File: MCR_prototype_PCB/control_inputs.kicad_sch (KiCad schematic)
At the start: 67 parts, among them J4 Conn_01x19_Pin, U1 74AHC165, U2 74AHC165

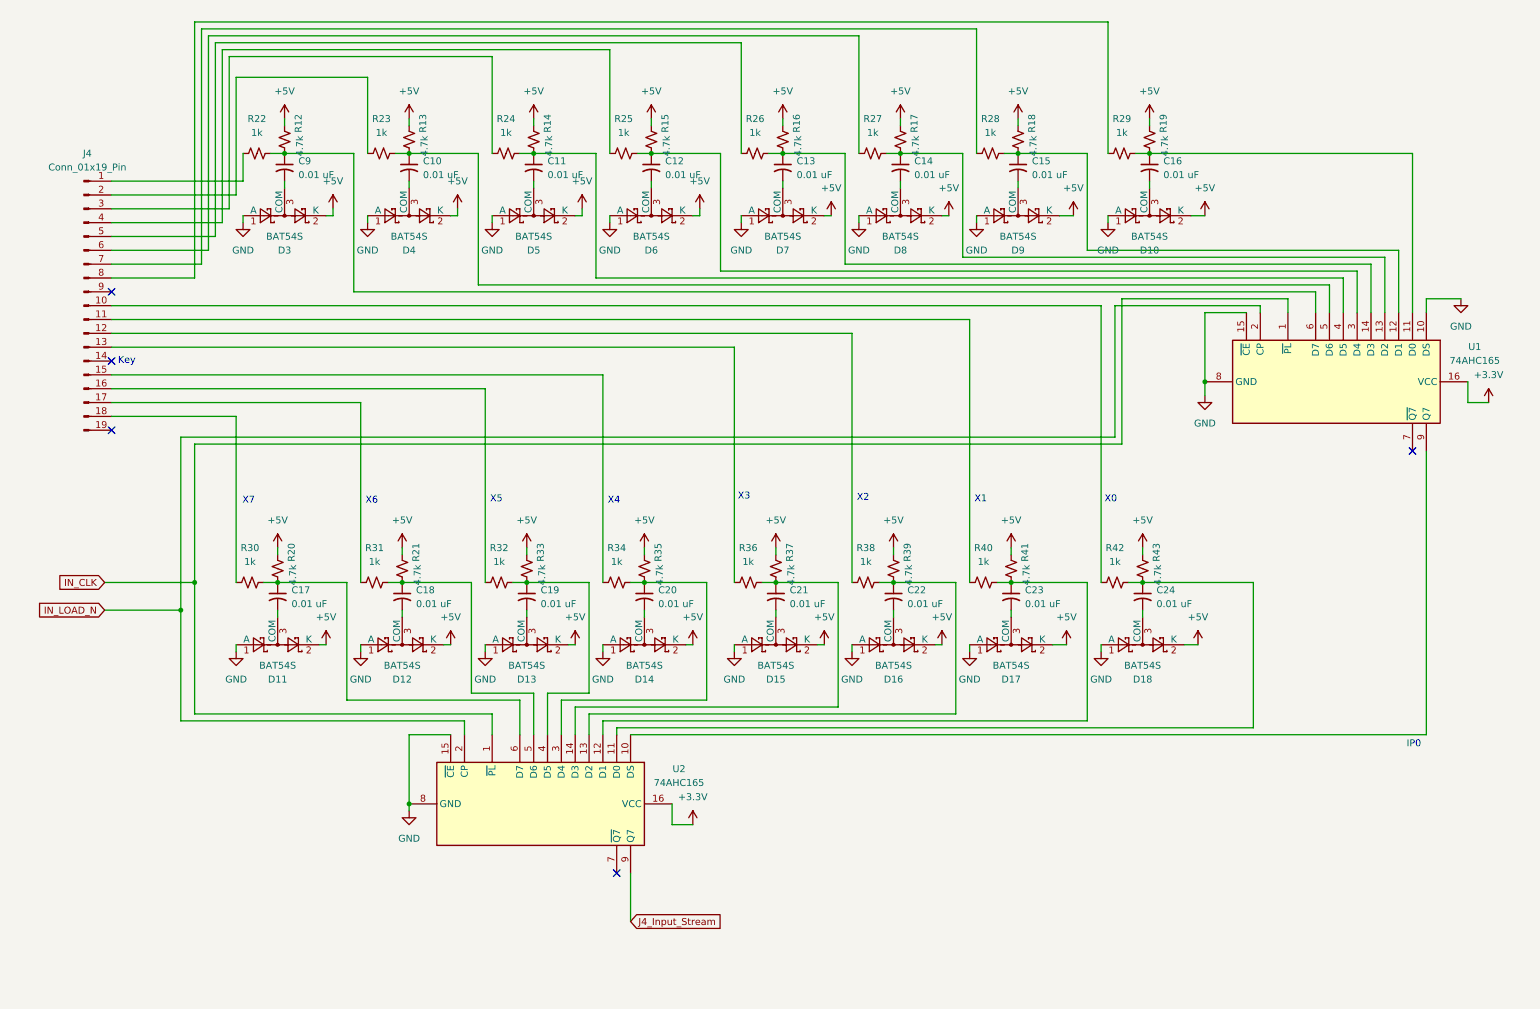
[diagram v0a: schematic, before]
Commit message: Updated 8/22/26
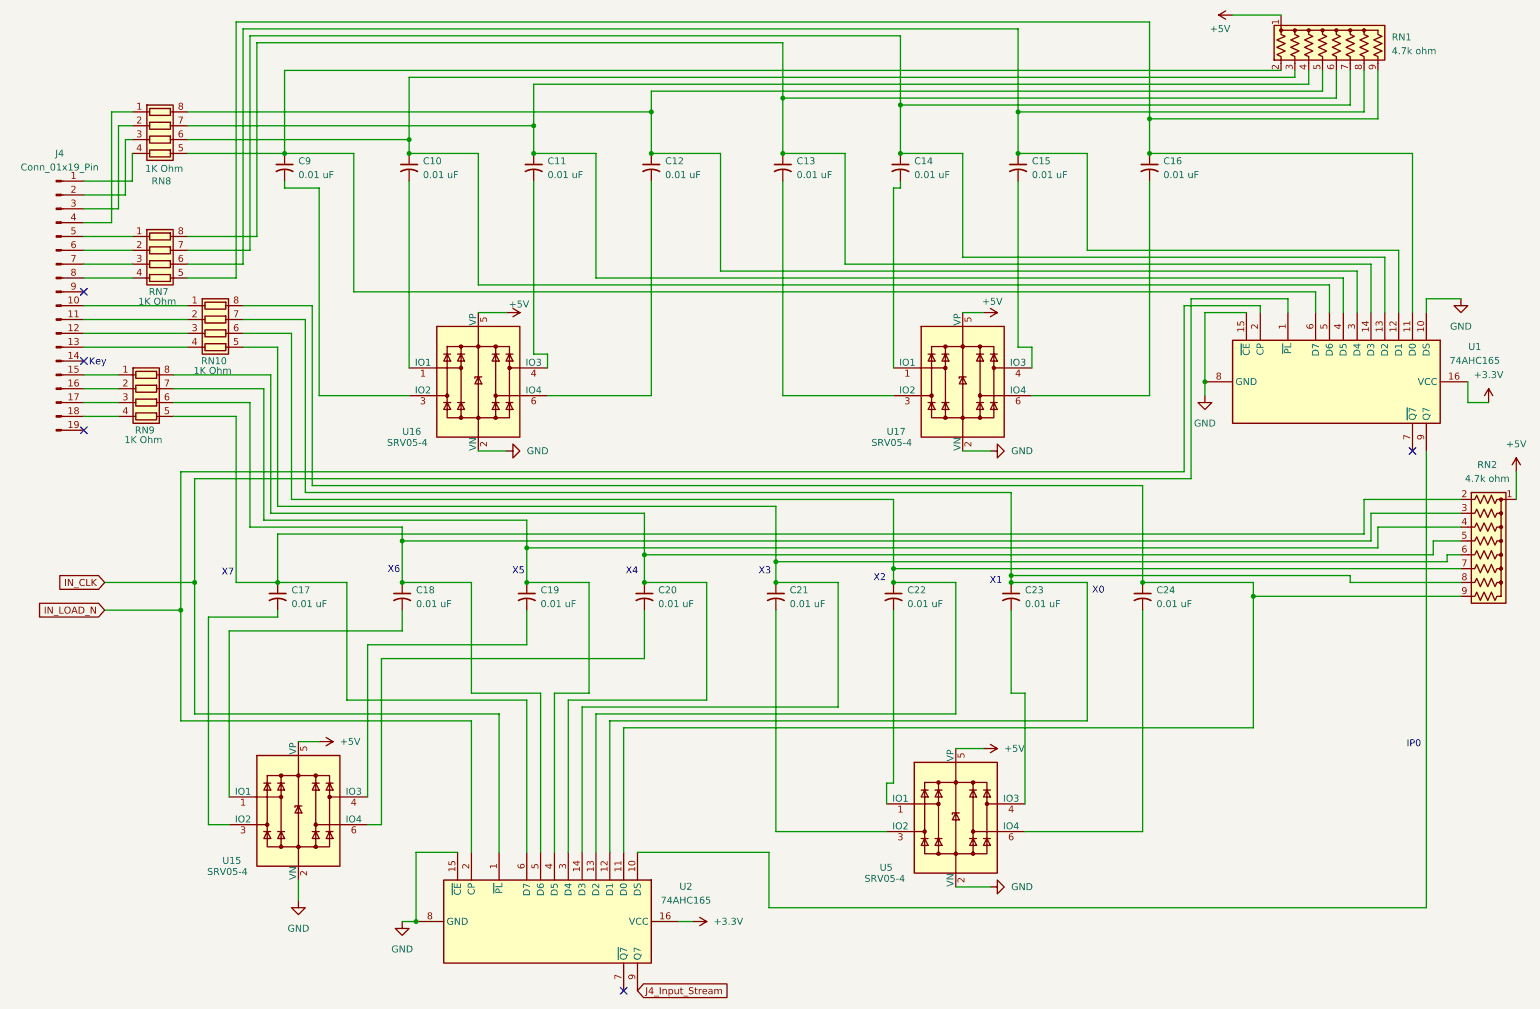
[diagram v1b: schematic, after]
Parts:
- removed D10, D11, D12, D13, D14, D15, D16, D17, D18, D3, D4, D5, D6, D7, D8, D9: BAT54S, Package_TO_SOT_SMD:SOT-23, symbol Diode:BAT54S
- removed R12, R13, R14, R15, R16, R17, R18, R19, R20, R21, R33, R35, R37, R39, R41, R43: 4.7k, Resistor_SMD:R_0805_2012Metric, symbol Device:R_Small_US
- removed R22, R23, R24, R25, R26, R27, R28, R29, R30, R31, R32, R34, R36, R38, R40, R42: 1k, Resistor_SMD:R_0805_2012Metric, symbol Device:R_Small_US
- added RN1, RN2: 4.7k ohm, Resistor_THT:R_Array_SIP9, symbol Device:R_Network08_US
- added RN10, RN7, RN8, RN9: 1K Ohm, Resistor_SMD:R_Array_Convex_4x0603, symbol Device:R_Pack04
- added U15, U16, U17, U5: SRV05-4, Package_TO_SOT_SMD:SOT-23-6, symbol Power_Protection:SRV05-4
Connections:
- net +5V: now also RN1.1 (common), RN2.1 (common), U15.5 (VP), U16.5 (VP), U17.5 (VP), U5.5 (VP)
- net GND: now also U15.2 (VN), U16.2 (VN), U17.2 (VN), U5.2 (VN)
- net at C15.1, U1.12 (D1): now also RN1.8 (R7), RN7.6 (R3.2)
- net at C15.2: now also U17.4 (IO3)
- net at C18.2: now also U15.1 (IO1)
- net at C17.1, U2.6 (D7): now also RN2.2 (R1), RN9.5 (R4.2)
- net at J4.18 (Pin_18): now also RN9.4 (R4.1)
- net at C23.1, U2.12 (D1): now also RN10.7 (R2.2), RN2.8 (R7)
- net at J4.11 (Pin_11): now also RN10.2 (R2.1)
- net at C18.1, U2.5 (D6): now also RN2.3 (R2), RN9.6 (R3.2)
- net at C16.1, U1.11 (D0): now also RN1.9 (R8), RN7.5 (R4.2)
- net at C16.2: now also U17.6 (IO4)
- net at C10.1, U1.5 (D6): now also RN1.3 (R2), RN8.6 (R3.2)
- net at C10.2: now also U16.1 (IO1)
- net at C13.1, U1.14 (D3): now also RN1.6 (R5), RN7.8 (R1.2)
- net at J4.5 (Pin_5): now also RN7.1 (R1.1)
- net at J4.8 (Pin_8): now also RN7.4 (R4.1)
- net at C24.1, U2.11 (D0): now also RN10.8 (R1.2), RN2.9 (R8)
- net at C22.1, U2.13 (D2): now also RN10.6 (R3.2), RN2.7 (R6)
- net at C21.1, U2.14 (D3): now also RN10.5 (R4.2), RN2.6 (R5)
- net at C20.1, U2.3 (D4): now also RN2.5 (R4), RN9.8 (R1.2)
- net at C19.1, U2.4 (D5): now also RN2.4 (R3), RN9.7 (R2.2)
- net at J4.13 (Pin_13): now also RN10.4 (R4.1)
- net at J4.16 (Pin_16): now also RN9.2 (R2.1)
- net at C12.1, U1.3 (D4): now also RN1.5 (R4), RN8.8 (R1.2)
- net at C12.2: now also U16.6 (IO4)
- net at C9.2: now also U16.3 (IO2)
- net at C17.2: now also U15.3 (IO2)
- net at C20.2: now also U15.6 (IO4)
- net at J4.2 (Pin_2): now also RN8.3 (R3.1)
- net at C11.1, U1.4 (D5): now also RN1.4 (R3), RN8.7 (R2.2)
- net at J4.3 (Pin_3): now also RN8.2 (R2.1)
- net at C19.2: now also U15.4 (IO3)
- net at J4.10 (Pin_10): now also RN10.1 (R1.1)
- net at C11.2: now also U16.4 (IO3)
- net at C9.1, U1.6 (D7): now also RN1.2 (R1), RN8.5 (R4.2)
- net at C24.2: now also U5.6 (IO4)
- net at C14.2: now also U17.1 (IO1)
- net at J4.17 (Pin_17): now also RN9.3 (R3.1)
- net at C14.1, U1.13 (D2): now also RN1.7 (R6), RN7.7 (R2.2)
- net at J4.7 (Pin_7): now also RN7.3 (R3.1)
- net at C21.2: now also U5.3 (IO2)
- net at J4.1 (Pin_1): now also RN8.4 (R4.1)
- net at J4.12 (Pin_12): now also RN10.3 (R3.1)
- net at J4.15 (Pin_15): now also RN9.1 (R1.1)
- net at J4.4 (Pin_4): now also RN8.1 (R1.1)
- net at J4.6 (Pin_6): now also RN7.2 (R2.1)
- net at C23.2: now also U5.4 (IO3)
- net at C13.2: now also U17.3 (IO2)
- net at C22.2: now also U5.1 (IO1)
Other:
- moved on the sheet: J4, U2
